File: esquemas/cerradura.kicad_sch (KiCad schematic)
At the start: 13 parts, among them J1 Conn_02x20_Odd_Even, J10 drv882x_righ_socket, J11 2n2222, J13 bornes_motor, J14 bornes_buzzer, J2 Conn_02x20_Odd_Even, J3 esp32_c3_right_socket, J4 num_keypad, J5 esp32_c3_left_socket, J6 R305_sensor, J7 RC522_sensor, J8 ssd1306_dsp, J9 drv882x_left_socket

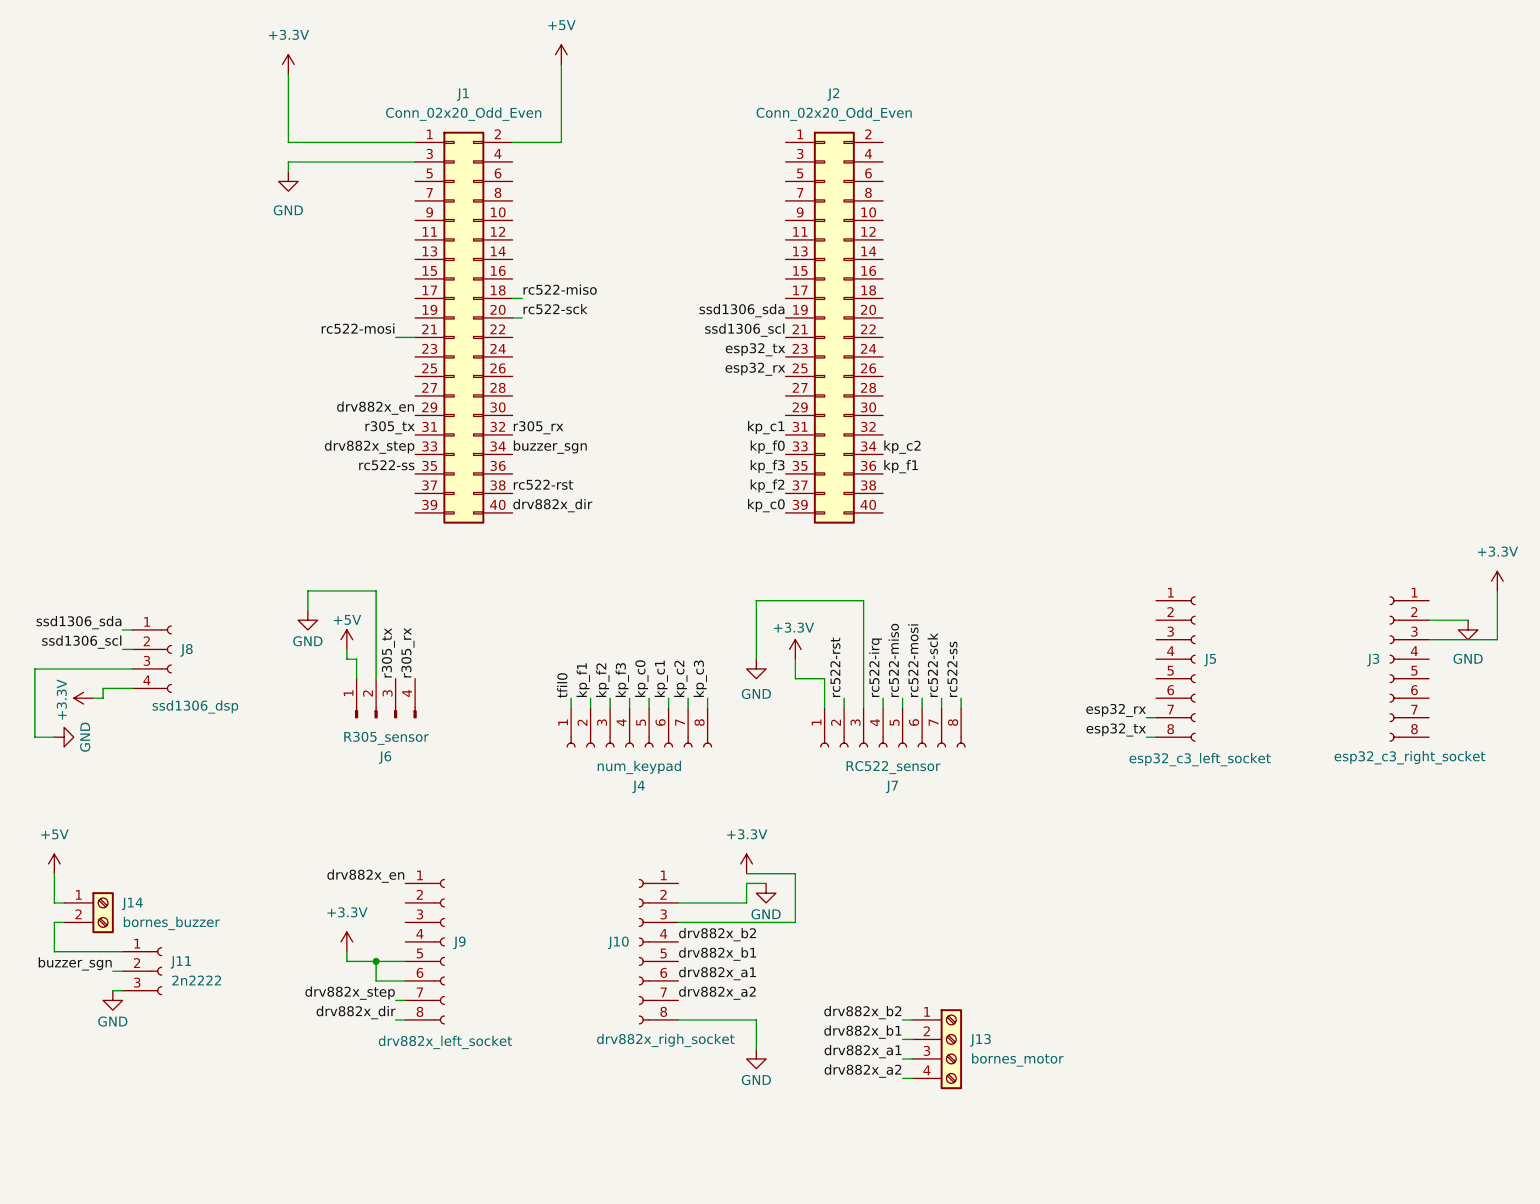
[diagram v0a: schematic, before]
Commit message: cambios dispositivos
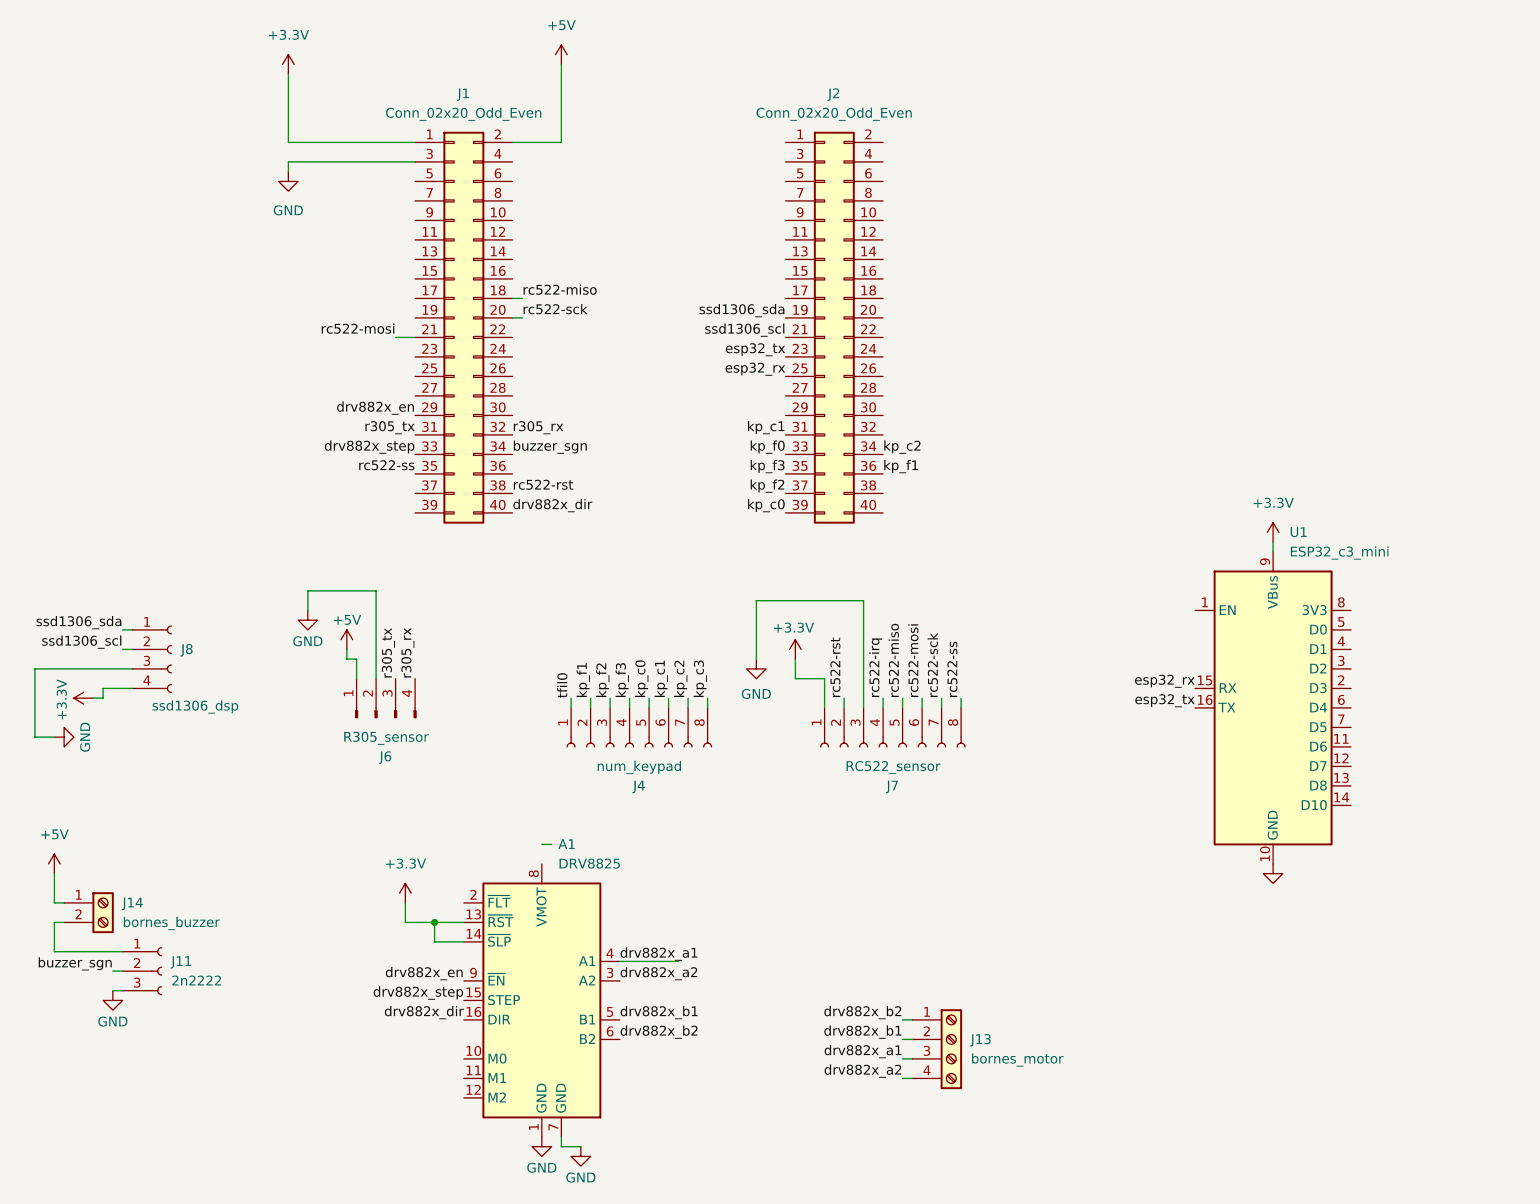
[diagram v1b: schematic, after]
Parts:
- removed J10: drv882x_righ_socket, Connector_Harwin:Harwin_M20-89008xx_1x08_P2.54mm_Horizontal, symbol Connector:Conn_01x08_Socket
- removed J3: esp32_c3_right_socket, Connector_Harwin:Harwin_M20-89008xx_1x08_P2.54mm_Horizontal, symbol Connector:Conn_01x08_Socket
- removed J5: esp32_c3_left_socket, Connector_Harwin:Harwin_M20-89008xx_1x08_P2.54mm_Horizontal, symbol Connector:Conn_01x08_Socket
- removed J9: drv882x_left_socket, Connector_Harwin:Harwin_M20-89008xx_1x08_P2.54mm_Horizontal, symbol Connector:Conn_01x08_Socket
- added A1: DRV8825, Module:Pololu_Breakout-16_15.2x20.3mm, symbol Driver_Motor:Pololu_Breakout_DRV8825
- added U1: ESP32_c3_mini, RF_Module:WEMOS_C3_mini, symbol RF_Module:WEMOS_C3_mini
- J11: footprint Connector_Harwin:Harwin_M20-89003xx_1x03_P2.54mm_Horizontal -> Connector_PinHeader_2.54mm:PinHeader_1x03_P2.54mm_Vertical
- J4, J7: footprint Connector_Harwin:Harwin_M20-89008xx_1x08_P2.54mm_Horizontal -> Connector_PinHeader_2.54mm:PinHeader_1x08_P2.54mm_Vertical
- J8: footprint Connector_Harwin:Harwin_M20-89004xx_1x04_P2.54mm_Horizontal -> Connector_PinSocket_2.54mm:PinSocket_1x04_P2.54mm_Vertical
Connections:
- net +3.3V: now also A1.13 (~{RST}), A1.14 (~{SLP}), U1.9 (VBus)
- net GND: now also A1.1 (GND), A1.7 (GND), U1.10 (GND)
- net drv882x_a1: now also A1.4 (A1)
- net drv882x_a2: now also A1.3 (A2)
- net drv882x_b1: now also A1.5 (B1)
- net drv882x_b2: now also A1.6 (B2)
- net drv882x_dir: now also A1.16 (DIR)
- net drv882x_en: now also A1.9 (~{EN})
- net drv882x_step: now also A1.15 (STEP)
- net esp32_rx: now also U1.15 (RX)
- net esp32_tx: now also U1.16 (TX)
